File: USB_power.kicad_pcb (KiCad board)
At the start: 2 copper layers, 20 parts, among them J1 PWR_IN, J2 USB_A_Stacked, J3 Power_check, J4 USB_C_Receptacle_USB2.0_16P

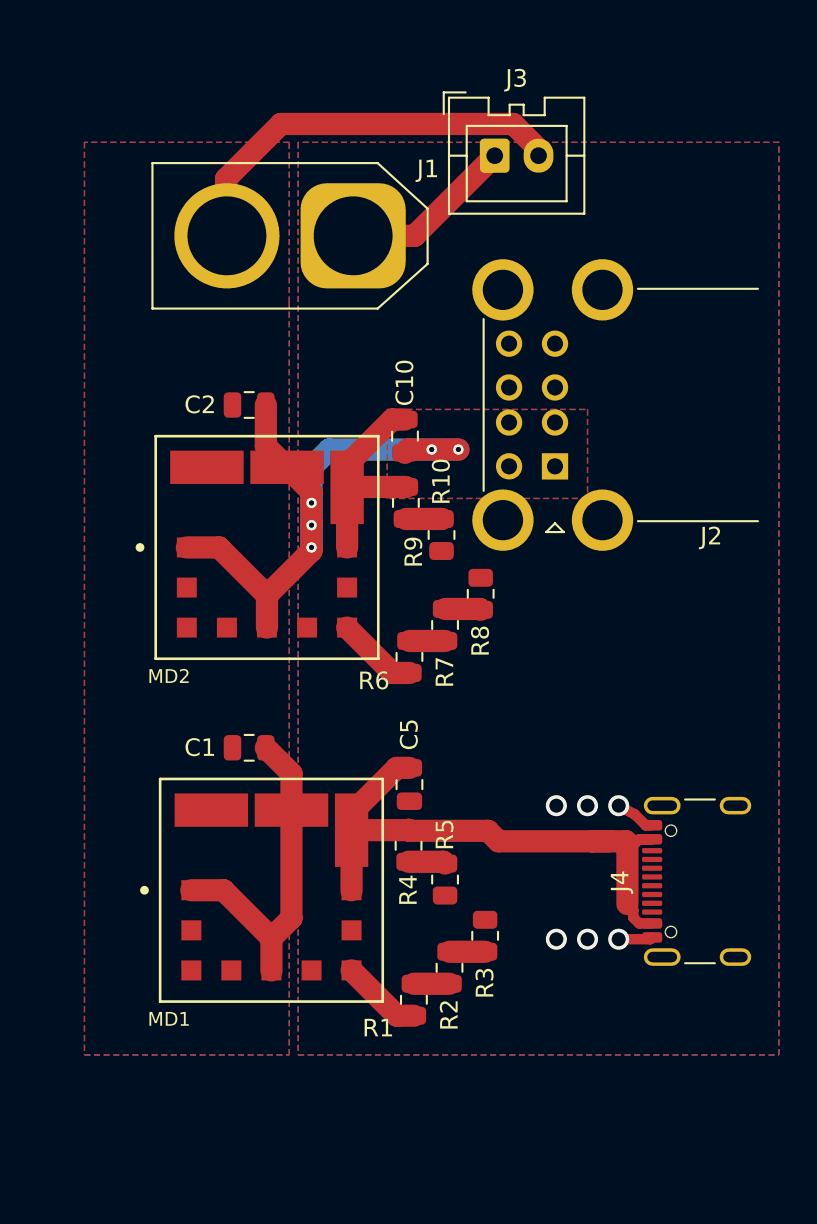
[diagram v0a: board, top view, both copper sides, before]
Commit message: 穴あけなど
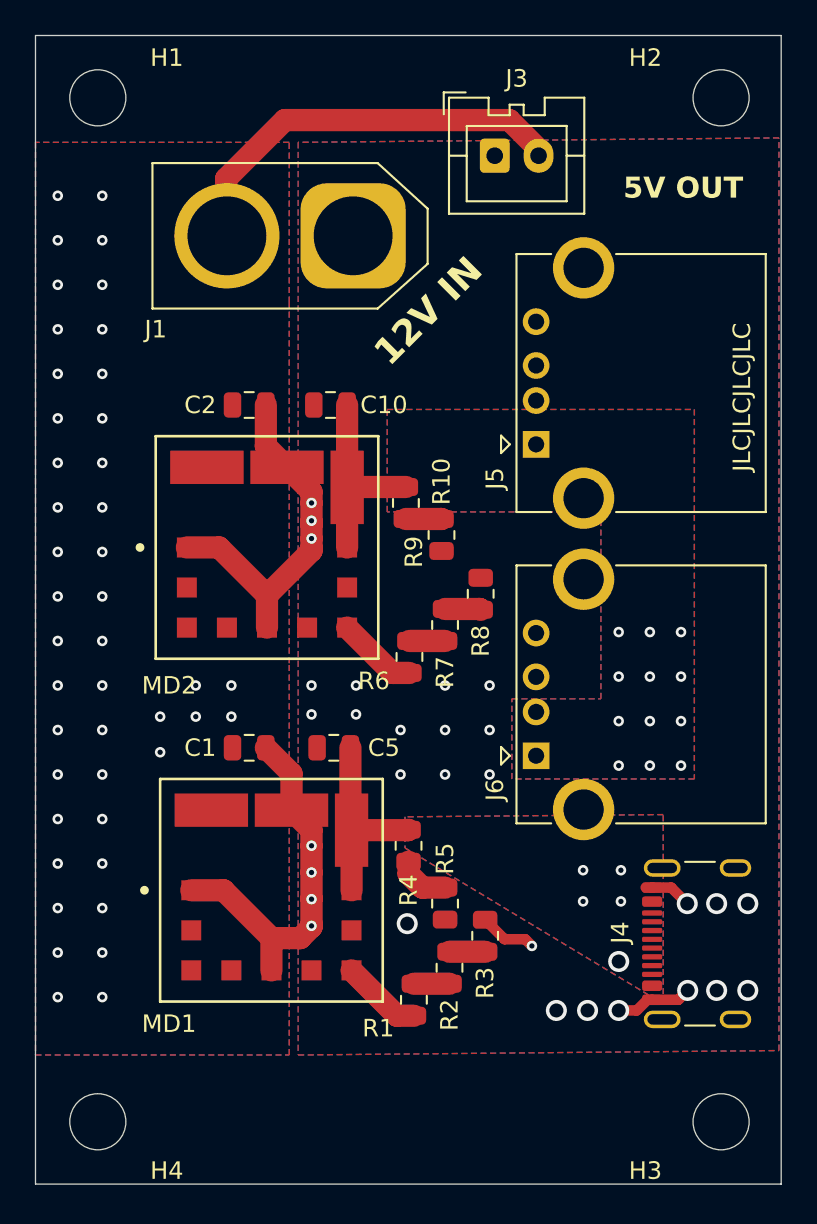
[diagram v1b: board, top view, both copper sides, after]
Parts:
- removed J2: USB_A_Stacked, Connector_USB:USB_A_CUI_UJ2-ADH-TH_Horizontal_Stacked
- added H1: MountingHole, MountingHole:MountingHole_3.2mm_M3, F.Cu at (43.7, 54.4)
- added H2: MountingHole, MountingHole:MountingHole_3.2mm_M3, F.Cu at (79.2, 54.4)
- added H3: MountingHole, MountingHole:MountingHole_3.2mm_M3, F.Cu at (79.2, 112.8)
- added H4: MountingHole, MountingHole:MountingHole_3.2mm_M3, F.Cu at (43.7, 112.8)
- added J5: USB_A, Connector_USB:USB_A_CONNFLY_DS1095-WNR0, F.Cu at (68.7, 74.1)
- added J6: USB_A, Connector_USB:USB_A_CONNFLY_DS1095-WNR0, F.Cu at (68.7, 91.9)
- moved C5 4.80 mm to (57.1, 91.4), turned to 180 degrees
- moved C10 4.61 mm to (57.0, 71.9), turned to 180 degrees
- moved J4 3.56 mm to (79.0, 102.6)
- moved R5 1.37 mm to (63.5, 100.3)
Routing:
- net +5V: track 33.7 -> 12.4 mm, vias 0 -> 5
- net GND: track 70.3 -> 52.4 mm, vias 11 -> 30
- net Net-(R4-Pad2): track 2.12 -> 3.10 mm
- net +5VP: track 12.5 -> 11.5 mm, vias 0 -> 12
- net +BATT: track 23.3 -> 23.5 mm, vias 0 -> 44
- added copper zone on B.Cu, net +5V
- added copper zone on F.Cu, net +5V
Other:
- board outline added: 42.5 x 65.5 mm
- board text added: "12V IN"
- board text added: "5V OUT"
- board text added: "JLCJLCJLCJLC"
